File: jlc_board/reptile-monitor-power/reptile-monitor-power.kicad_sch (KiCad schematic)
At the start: 10 parts, among them J1 AC_IN, J2 LOAD_2, J3 LOAD_1, J4 POWER CONN, K1 ALDP105W, K2 ALDP105W, U1 NUD3105DMT1G

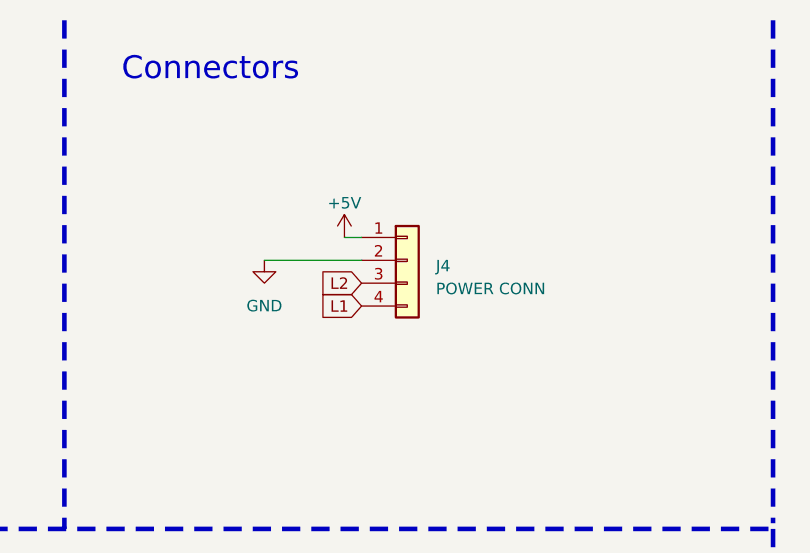
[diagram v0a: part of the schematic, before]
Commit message: updates
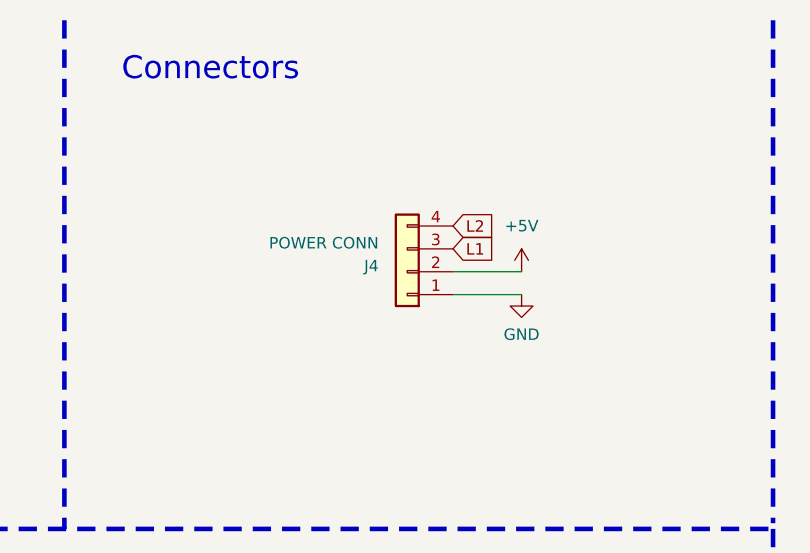
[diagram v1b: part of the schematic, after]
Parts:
- F1: footprint SamacSys_Parts:TO508P400X850X850-2P -> reptile-monitor-power:TO508P400X850X850-2P
- J1, J2, J3: footprint SamacSys_Parts:128340212 -> reptile-monitor-power:TE Connectivity PC Terminal Block 128340212
- J4: footprint Connector_PinHeader_2.54mm:PinHeader_1x04_P2.54mm_Vertical -> reptile-monitor-power:PinHeader_1x04_P2.54mm_Vertical
- PS1: footprint Converter_ACDC:Converter_ACDC_HiLink_HLK-PMxx -> reptile-monitor-power:Converter_ACDC_HiLink_HLK-PMxx
- RV1: footprint Varistor:RV_Disc_D7mm_W3.4mm_P5mm -> reptile-monitor-power:RV_Disc_D7mm_W3.4mm_P5mm
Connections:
- net +5V: now also J4.2 (Pin_2); no longer J4.1 (Pin_1)
- net GND: now also J4.1 (Pin_1); no longer J4.2 (Pin_2)
- net L1: now also J4.3 (Pin_3); no longer J4.4 (Pin_4)
- net L2: now also J4.4 (Pin_4); no longer J4.3 (Pin_3)
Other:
- moved on the sheet: J4
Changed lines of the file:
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@@
-(kicad_sch (version 20210406) (generator eeschema)
+(kicad_sch (version 20210621) (generator eeschema)
   (paper "A4")
   (junction (at 27.94 39.37) (diameter 0.9144) (color 0 0 0 0))
@@
     (stroke (width 0) (type solid) (color 0 0 0 0))
   )
-  (wire (pts (xy 120.65 39.37) (xy 131.445 39.37))
-    (stroke (width 0) (type solid) (color 0 0 0 0))
-  )
-  (wire (pts (xy 129.54 36.83) (xy 131.445 36.83))
+  (wire (pts (xy 141.605 40.64) (xy 149.225 40.64))
+    (stroke (width 0) (type solid) (color 0 0 0 0))
+  )
+  (wire (pts (xy 141.605 43.18) (xy 149.225 43.18))
     (stroke (width 0) (type solid) (color 0 0 0 0))
   )
@@
     )
   )
-  (global_label "L2" (shape input) (at 131.445 41.91 180) (fields_autoplaced)
-    (effects (font (size 1.27 1.27)) (justify right))
-    (property "Intersheet References" "${INTERSHEET_REFS}" (id 0) (at 126.7943 41.8306 0)
-      (effects (font (size 1.27 1.27)) (justify right) hide)
-    )
-  )
-  (global_label "L1" (shape input) (at 131.445 44.45 180) (fields_autoplaced)
-    (effects (font (size 1.27 1.27)) (justify right))
-    (property "Intersheet References" "${INTERSHEET_REFS}" (id 0) (at 126.7943 44.3706 0)
-      (effects (font (size 1.27 1.27)) (justify right) hide)
+  (global_label "L2" (shape input) (at 141.605 35.56 0) (fields_autoplaced)
+    (effects (font (size 1.27 1.27)) (justify left))
+    (property "Intersheet References" "${INTERSHEET_REFS}" (id 0) (at 146.2557 35.6394 0)
+      (effects (font (size 1.27 1.27)) (justify left) hide)
+    )
+  )
+  (global_label "L1" (shape input) (at 141.605 38.1 0) (fields_autoplaced)
+    (effects (font (size 1.27 1.27)) (justify left))
+    (property "Intersheet References" "${INTERSHEET_REFS}" (id 0) (at 146.2557 38.1794 0)
+      (effects (font (size 1.27 1.27)) (justify left) hide)
     )
   )
@@
     (pin "1")
   )
-  (symbol (lib_id "power:+5V") (at 129.54 36.83 0) (unit 1)
-    (in_bom yes) (on_board yes) (fields_autoplaced)
-    (property "Reference" "#PWR0106" (id 0) (at 129.54 40.64 0)
-      (effects (font (size 1.27 1.27)) hide)
-    )
-    (property "Value" "+5V" (id 1) (at 129.54 33.02 0))
-    (property "Footprint" "" (id 2) (at 129.54 36.83 0)
-      (effects (font (size 1.27 1.27)) hide)
-    )
-    (property "Datasheet" "" (id 3) (at 129.54 36.83 0)
+  (symbol (lib_id "power:+5V") (at 149.225 40.64 0) (unit 1)
+    (in_bom yes) (on_board yes) (fields_autoplaced)
+    (property "Reference" "#PWR0106" (id 0) (at 149.225 44.45 0)
+      (effects (font (size 1.27 1.27)) hide)
+    )
+    (property "Value" "+5V" (id 1) (at 149.225 35.56 0))
+    (property "Footprint" "" (id 2) (at 149.225 40.64 0)
+      (effects (font (size 1.27 1.27)) hide)
+    )
+    (property "Datasheet" "" (id 3) (at 149.225 40.64 0)
       (effects (font (size 1.27 1.27)) hide)
     )
@@
     (pin "1")
   )
-  (symbol (lib_id "power:GND") (at 120.65 39.37 0) (unit 1)
-    (in_bom yes) (on_board yes) (fields_autoplaced)
-    (property "Reference" "#PWR0101" (id 0) (at 120.65 45.72 0)
-      (effects (font (size 1.27 1.27)) hide)
-    )
-    (property "Value" "GND" (id 1) (at 120.65 44.45 0))
-    (property "Footprint" "" (id 2) (at 120.65 39.37 0)
-      (effects (font (size 1.27 1.27)) hide)
-    )
-    (property "Datasheet" "" (id 3) (at 120.65 39.37 0)
+  (symbol (lib_id "power:GND") (at 149.225 43.18 0) (unit 1)
+    (in_bom yes) (on_board yes)
+    (property "Reference" "#PWR0101" (id 0) (at 149.225 49.53 0)
+      (effects (font (size 1.27 1.27)) hide)
+    )
+    (property "Value" "GND" (id 1) (at 149.225 47.625 0))
+    (property "Footprint" "" (id 2) (at 149.225 43.18 0)
+      (effects (font (size 1.27 1.27)) hide)
+    )
+    (property "Datasheet" "" (id 3) (at 149.225 43.18 0)
       (effects (font (size 1.27 1.27)) hide)
     )
@@
     (property "Reference" "J1" (id 0) (at 21.717 34.29 0))
     (property "Value" "AC_IN" (id 1) (at 21.717 36.83 0))
-    (property "Footprint" "SamacSys_Parts:128340212" (id 2) (at 19.685 39.37 0)
+    (property "Footprint" "reptile-monitor-power:TE Connectivity PC Terminal Block 128340212" (id 2) (at 19.685 39.37 0)
       (effects (font (size 1.27 1.27)) hide)
     )
@@
       (effects (font (size 1.27 1.27)) (justify left))
     )
-    (property "Footprint" "SamacSys_Parts:128340212" (id 2) (at 102.235 91.44 0)
+    (property "Footprint" "reptile-monitor-power:TE Connectivity PC Terminal Block 128340212" (id 2) (at 102.235 91.44 0)
       (effects (font (size 1.27 1.27)) hide)
     )
@@
       (effects (font (size 1.27 1.27)) (justify left))
     )
-    (property "Footprint" "SamacSys_Parts:128340212" (id 2) (at 102.235 109.855 0)
+    (property "Footprint" "reptile-monitor-power:TE Connectivity PC Terminal Block 128340212" (id 2) (at 102.235 109.855 0)
       (effects (font (size 1.27 1.27)) hide)
     )
@@
     (property "Reference" "RV1" (id 0) (at 51.435 47.625 90))
     (property "Value" "Varistor" (id 1) (at 51.435 45.72 90))
-    (property "Footprint" "Varistor:RV_Disc_D7mm_W3.4mm_P5mm" (id 2) (at 51.435 43.688 90)
+    (property "Footprint" "reptile-monitor-power:RV_Disc_D7mm_W3.4mm_P5mm" (id 2) (at 51.435 43.688 90)
       (effects (font (size 1.27 1.27)) hide)
     )
@@
     (property "Reference" "F1" (id 0) (at 40.005 34.29 0))
     (property "Value" "39208000440" (id 1) (at 40.005 36.83 0))
-    (property "Footprint" "SamacSys_Parts:TO508P400X850X850-2P" (id 2) (at 34.925 38.1 0)
+    (property "Footprint" "reptile-monitor-power:TO508P400X850X850-2P" (id 2) (at 34.925 38.1 0)
       (effects (font (size 1.27 1.27)) (justify left) hide)
     )
@@
     (pin "2")
   )
-  (symbol (lib_id "Connector_Generic:Conn_01x04") (at 136.525 39.37 0) (unit 1)
-    (in_bom yes) (on_board yes) (fields_autoplaced)
-    (property "Reference" "J4" (id 0) (at 139.7 40.0049 0)
+  (symbol (lib_id "Connector_Generic:Conn_01x04") (at 136.525 40.64 180) (unit 1)
+    (in_bom yes) (on_board yes) (fields_autoplaced)
+    (property "Reference" "J4" (id 0) (at 133.35 40.0051 0)
       (effects (font (size 1.27 1.27)) (justify left))
     )
-    (property "Value" "POWER CONN" (id 1) (at 139.7 42.5449 0)
+    (property "Value" "POWER CONN" (id 1) (at 133.35 37.4651 0)
       (effects (font (size 1.27 1.27)) (justify left))
     )
-    (property "Footprint" "Connector_PinHeader_2.54mm:PinHeader_1x04_P2.54mm_Vertical" (id 2) (at 136.525 39.37 0)
-      (effects (font (size 1.27 1.27)) hide)
-    )
-    (property "Datasheet" "~" (id 3) (at 136.525 39.37 0)
+    (property "Footprint" "reptile-monitor-power:PinHeader_1x04_P2.54mm_Vertical" (id 2) (at 136.525 40.64 0)
+      (effects (font (size 1.27 1.27)) hide)
+    )
+    (property "Datasheet" "~" (id 3) (at 136.525 40.64 0)
       (effects (font (size 1.27 1.27)) hide)
     )
@@
     (property "Reference" "PS1" (id 0) (at 71.755 33.655 0))
     (property "Value" "HLK-PM01" (id 1) (at 71.755 36.195 0))
-    (property "Footprint" "Converter_ACDC:Converter_ACDC_HiLink_HLK-PMxx" (id 2) (at 71.755 49.53 0)
+    (property "Footprint" "reptile-monitor-power:Converter_ACDC_HiLink_HLK-PMxx" (id 2) (at 71.755 49.53 0)
       (effects (font (size 1.27 1.27)) hide)
     )
@@
     )
     (path "/65937042-b870-4bb1-8295-d42aeb83a7dc"
-      (reference "F1") (unit 1) (value "39208000440") (footprint "SamacSys_Parts:TO508P400X850X850-2P")
+      (reference "F1") (unit 1) (value "39208000440") (footprint "reptile-monitor-power:TO508P400X850X850-2P")
     )
     (path "/b1c76bd5-4103-49d9-9263-d65f3e68d243"
-      (reference "J1") (unit 1) (value "AC_IN") (footprint "SamacSys_Parts:128340212")
+      (reference "J1") (unit 1) (value "AC_IN") (footprint "reptile-monitor-power:TE Connectivity PC Terminal Block 128340212")
     )
     (path "/dfdc75d1-1c52-4480-9f16-a64c1f1a624d"
-      (reference "J2") (unit 1) (value "LOAD_2") (footprint "SamacSys_Parts:128340212")
+      (reference "J2") (unit 1) (value "LOAD_2") (footprint "reptile-monitor-power:TE Connectivity PC Terminal Block 128340212")
     )
     (path "/b80ad536-9d44-457f-ae45-467e55d21e7b"
-      (reference "J3") (unit 1) (value "LOAD_1") (footprint "SamacSys_Parts:128340212")
+      (reference "J3") (unit 1) (value "LOAD_1") (footprint "reptile-monitor-power:TE Connectivity PC Terminal Block 128340212")
     )
     (path "/f7417c66-6cf1-4a1c-906a-bac3e603a63d"
-      (reference "J4") (unit 1) (value "POWER CONN") (footprint "Connector_PinHeader_2.54mm:PinHeader_1x04_P2.54mm_Vertical")
+      (reference "J4") (unit 1) (value "POWER CONN") (footprint "reptile-monitor-power:PinHeader_1x04_P2.54mm_Vertical")
     )
     (path "/70a37dcc-1d6f-4c53-acc5-ce6d37b633d7"
@@
     )
     (path "/874a92e5-5fd4-4ca2-be27-4b579b7dff85"
-      (reference "PS1") (unit 1) (value "HLK-PM01") (footprint "Converter_ACDC:Converter_ACDC_HiLink_HLK-PMxx")
+      (reference "PS1") (unit 1) (value "HLK-PM01") (footprint "reptile-monitor-power:Converter_ACDC_HiLink_HLK-PMxx")
     )
     (path "/bc4c5b99-7501-44d0-833b-04f8a03ba133"
-      (reference "RV1") (unit 1) (value "Varistor") (footprint "Varistor:RV_Disc_D7mm_W3.4mm_P5mm")
+      (reference "RV1") (unit 1) (value "Varistor") (footprint "reptile-monitor-power:RV_Disc_D7mm_W3.4mm_P5mm")
     )
     (path "/80350614-fa47-45e4-8e74-7a2d58fd936a"
